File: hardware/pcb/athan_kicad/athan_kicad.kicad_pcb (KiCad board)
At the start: 2 copper layers, 183.5 x 127.1 mm, 27 parts, among them J1 USB_C_Receptacle_PowerOnly_6P, J2 AudioJack4, SW1 ui_select, SW2 ui_next, SW3 SW_SPST

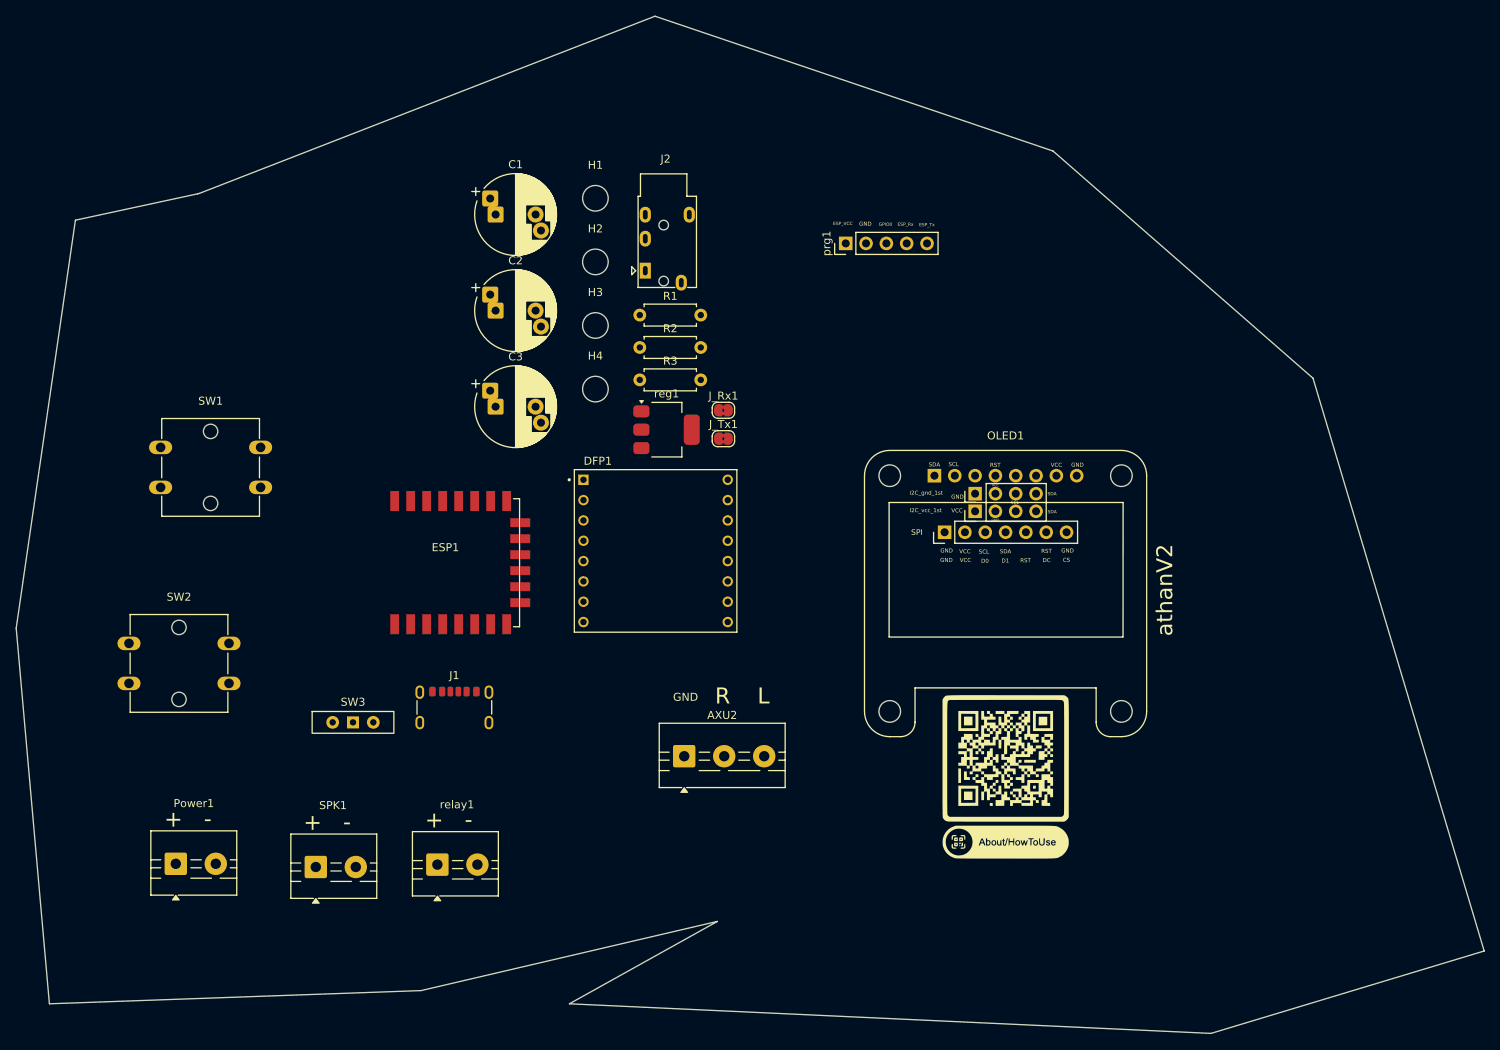
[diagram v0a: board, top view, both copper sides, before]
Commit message: PCB V2 in progress
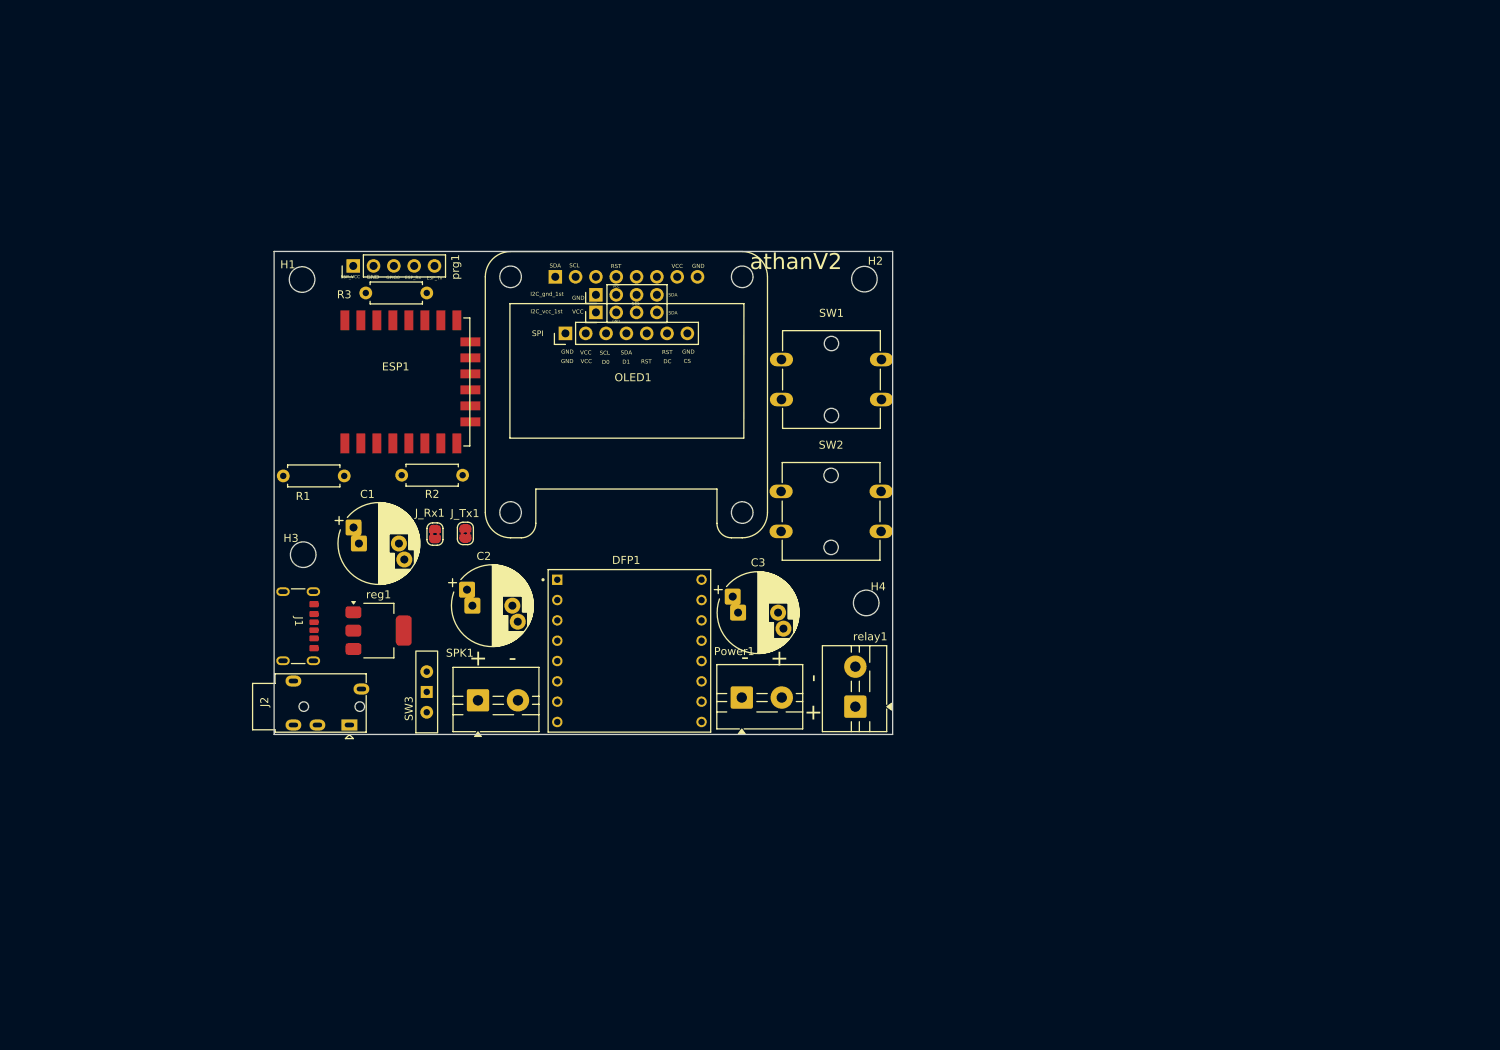
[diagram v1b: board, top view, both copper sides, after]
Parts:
- removed AXU2: Conn_01x03, TerminalBlock:TerminalBlock_MaiXu_MX126-5.0-03P_1x03_P5.00mm
- G***: moved to B.Cu
- moved SW2 83.7 mm to (122.3, 84.8)
- moved SW1 78.4 mm to (122.3, 68.4)
- moved Power1 73.7 mm to (117.3, 110.6)
- moved J2 67.8 mm to (68.3, 114.0), turned to 90 degrees
- moved prg1 61.6 mm to (68.8, 56.7)
- moved G*** 61.5 mm to (102.8, 81.6), turned to 180 degrees
- moved relay1 55.8 mm to (131.5, 111.8), turned to 90 degrees
- moved OLED1 53.5 mm to (94.0, 58.0)
- moved R1 48.9 mm to (60.0, 82.9)
- moved H3 46.4 mm to (62.5, 92.8)
- moved C1 44.5 mm to (69.5, 91.4)
- moved reg1 43.9 mm to (72.0, 102.2)
- moved H4 43.1 mm to (132.9, 98.8)
- moved C3 39.8 mm to (116.9, 100.0)
- moved J_Rx1 39.2 mm to (79.0, 90.2), turned to 90 degrees
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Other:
- board size 183.5 x 127.1 mm -> 77.3 x 60.4 mm
- board text removed: "L"
- board text removed: "R"
